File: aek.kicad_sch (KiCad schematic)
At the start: 242 parts, among them J1 Conn_01x04_MountingPin, SW1 SW_Push, U1 ATmega32U4-AU, U2 ATmega32U4-MU, Y1 16MHz

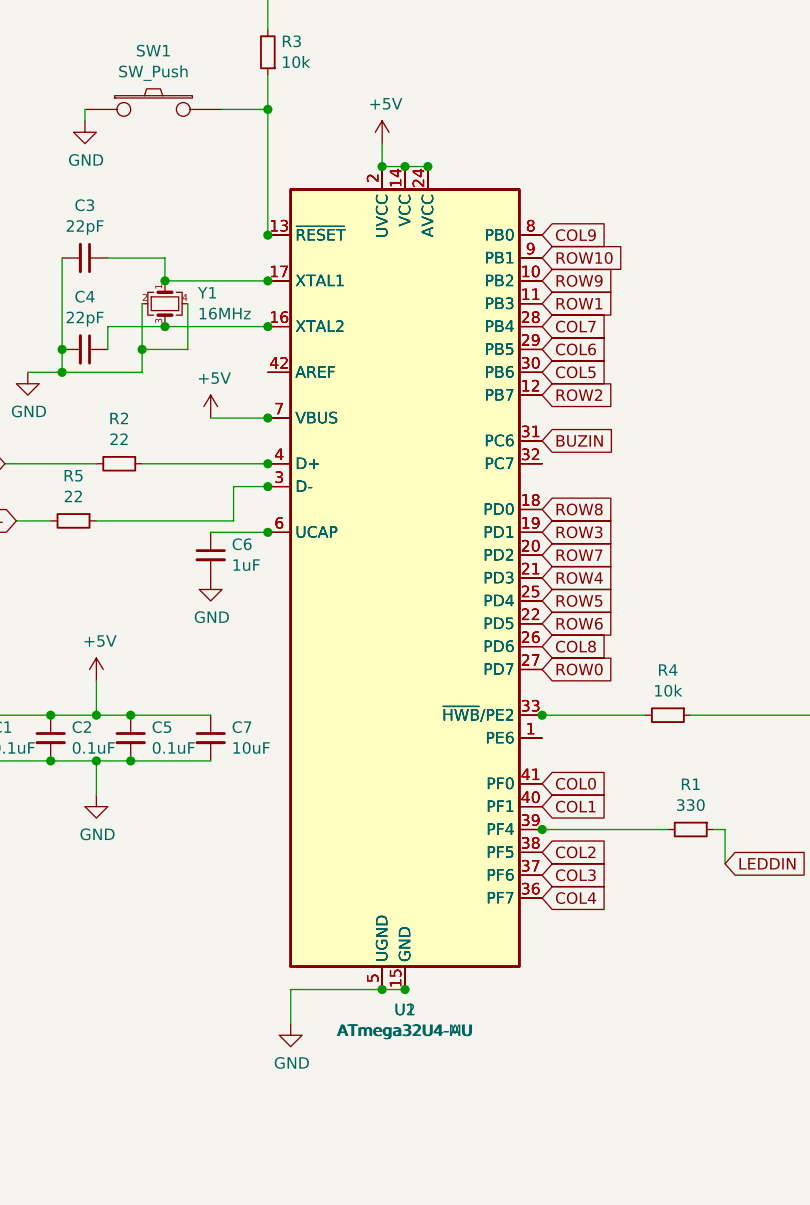
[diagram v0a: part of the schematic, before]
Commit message: cleanup
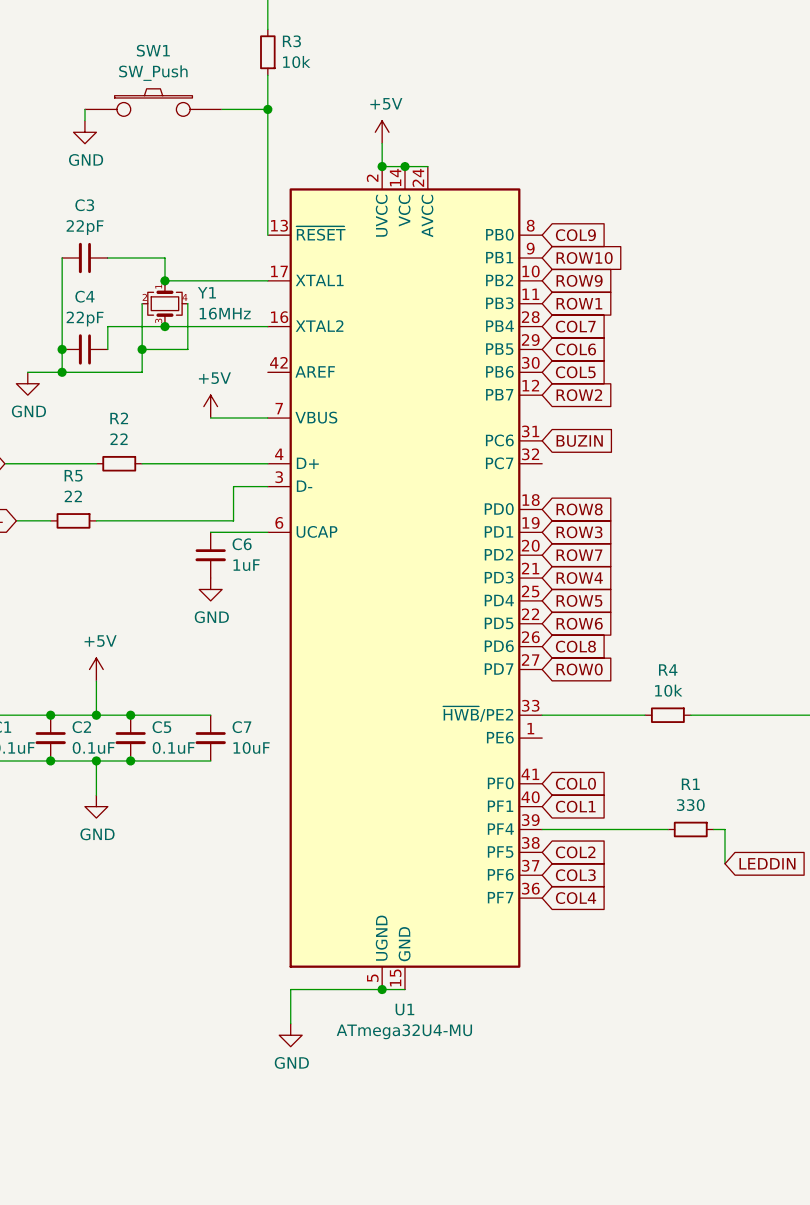
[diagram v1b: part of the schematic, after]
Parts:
- removed U1: ATmega32U4-AU, Package_QFP:TQFP-44_10x10mm_P0.8mm, symbol MCU_Microchip_ATmega:ATmega32U4-AU
- U1: renamed from U2; footprint Package_DFN_QFN:QFN-44-1EP_7x7mm_P0.5mm_EP5.2x5.2mm -> atmega32u4-au-and-mu:atmega32u4-mu-and-au
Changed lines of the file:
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@@
   (junction (at 39.37 59.69) (diameter 1.016) (color 0 0 0 0))
   (junction (at 50.8 35.56) (diameter 1.016) (color 0 0 0 0))
-  (junction (at 50.8 49.53) (diameter 1.016) (color 0 0 0 0))
-  (junction (at 50.8 54.61) (diameter 1.016) (color 0 0 0 0))
-  (junction (at 50.8 59.69) (diameter 1.016) (color 0 0 0 0))
-  (junction (at 50.8 69.85) (diameter 1.016) (color 0 0 0 0))
-  (junction (at 50.8 74.93) (diameter 1.016) (color 0 0 0 0))
-  (junction (at 50.8 77.47) (diameter 1.016) (color 0 0 0 0))
-  (junction (at 50.8 82.55) (diameter 1.016) (color 0 0 0 0))
   (junction (at 63.5 41.91) (diameter 1.016) (color 0 0 0 0))
   (junction (at 63.5 133.35) (diameter 1.016) (color 0 0 0 0))
@@
   (junction (at 64.77 241.3) (diameter 1.016) (color 0 0 0 0))
   (junction (at 66.04 41.91) (diameter 1.016) (color 0 0 0 0))
-  (junction (at 66.04 133.35) (diameter 1.016) (color 0 0 0 0))
-  (junction (at 68.58 41.91) (diameter 1.016) (color 0 0 0 0))
-  (junction (at 81.28 102.87) (diameter 1.016) (color 0 0 0 0))
-  (junction (at 81.28 115.57) (diameter 1.016) (color 0 0 0 0))
   (junction (at 100.33 241.3) (diameter 1.016) (color 0 0 0 0))
   (junction (at 157.48 55.88) (diameter 1.016) (color 0 0 0 0))
@@
     (pin "4")
   )
-  (symbol (lib_id "MCU_Microchip_ATmega:ATmega32U4-AU") (at 66.04 87.63 0) (unit 1)
-    (in_bom yes) (on_board yes)
-    (property "Reference" "U1" (id 0) (at 66.04 135.6106 0))
-    (property "Value" "ATmega32U4-AU" (id 1) (at 66.04 137.922 0))
-    (property "Footprint" "Package_QFP:TQFP-44_10x10mm_P0.8mm" (id 2) (at 66.04 87.63 0)
-      (effects (font (size 1.27 1.27) italic) hide)
-    )
-    (property "Datasheet" "http://ww1.microchip.com/downloads/en/DeviceDoc/Atmel-7766-8-bit-AVR-ATmega16U4-32U4_Datasheet.pdf" (id 3) (at 66.04 87.63 0)
-      (effects (font (size 1.27 1.27)) hide)
-    )
-    (pin "1")
-    (pin "10")
-    (pin "11")
-    (pin "12")
-    (pin "13")
-    (pin "14")
-    (pin "15")
-    (pin "16")
-    (pin "17")
-    (pin "18")
-    (pin "19")
-    (pin "2")
-    (pin "20")
-    (pin "21")
-    (pin "22")
-    (pin "23")
-    (pin "24")
-    (pin "25")
-    (pin "26")
-    (pin "27")
-    (pin "28")
-    (pin "29")
-    (pin "3")
-    (pin "30")
-    (pin "31")
-    (pin "32")
-    (pin "33")
-    (pin "34")
-    (pin "35")
-    (pin "36")
-    (pin "37")
-    (pin "38")
-    (pin "39")
-    (pin "4")
-    (pin "40")
-    (pin "41")
-    (pin "42")
-    (pin "43")
-    (pin "44")
-    (pin "5")
-    (pin "6")
-    (pin "7")
-    (pin "8")
-    (pin "9")
-  )
   (symbol (lib_id "MCU_Microchip_ATmega:ATmega32U4-MU") (at 66.04 87.63 0) (unit 1)
     (in_bom yes) (on_board yes)
-    (property "Reference" "U2" (id 0) (at 66.04 135.6106 0))
+    (property "Reference" "U1" (id 0) (at 66.04 135.6106 0))
     (property "Value" "ATmega32U4-MU" (id 1) (at 66.04 137.922 0))
-    (property "Footprint" "Package_DFN_QFN:QFN-44-1EP_7x7mm_P0.5mm_EP5.2x5.2mm" (id 2) (at 66.04 87.63 0)
+    (property "Footprint" "atmega32u4-au-and-mu:atmega32u4-mu-and-au" (id 2) (at 66.04 87.63 0)
       (effects (font (size 1.27 1.27) italic) hide)
     )
@@
       (reference "SW_Z1") (unit 1) (value "MX-NoLED") (footprint "MX_Alps_Hybrid:MX-1U-NoLED")
     )
-    (path "/00000000-0000-0000-0000-0000611ebb71"
-      (reference "U1") (unit 1) (value "ATmega32U4-AU") (footprint "Package_QFP:TQFP-44_10x10mm_P0.8mm")
-    )
     (path "/2ccdb65d-62ed-42d5-acea-df4cedf22149"
-      (reference "U2") (unit 1) (value "ATmega32U4-MU") (footprint "Package_DFN_QFN:QFN-44-1EP_7x7mm_P0.5mm_EP5.2x5.2mm")
+      (reference "U1") (unit 1) (value "ATmega32U4-MU") (footprint "atmega32u4-au-and-mu:atmega32u4-mu-and-au")
     )
     (path "/00000000-0000-0000-0000-0000612269b2"

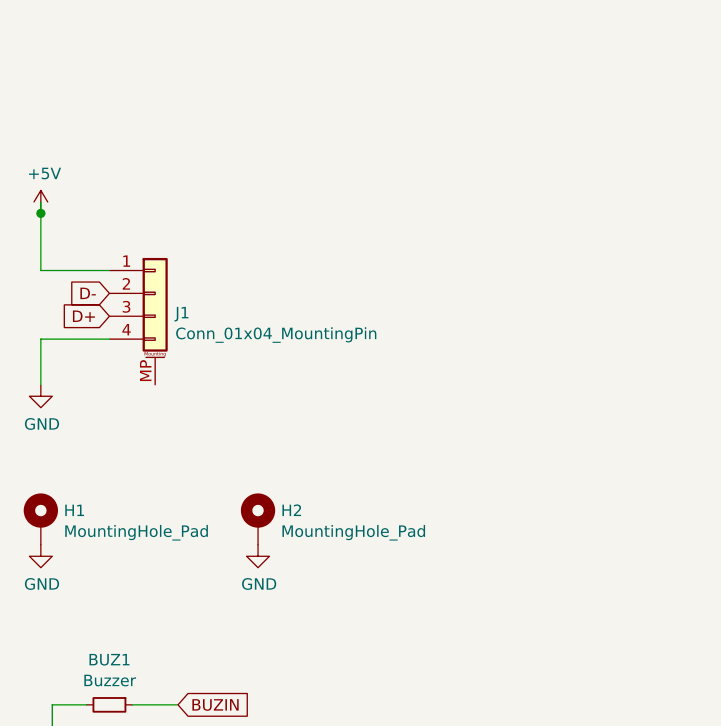
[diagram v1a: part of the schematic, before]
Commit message: bug fixes
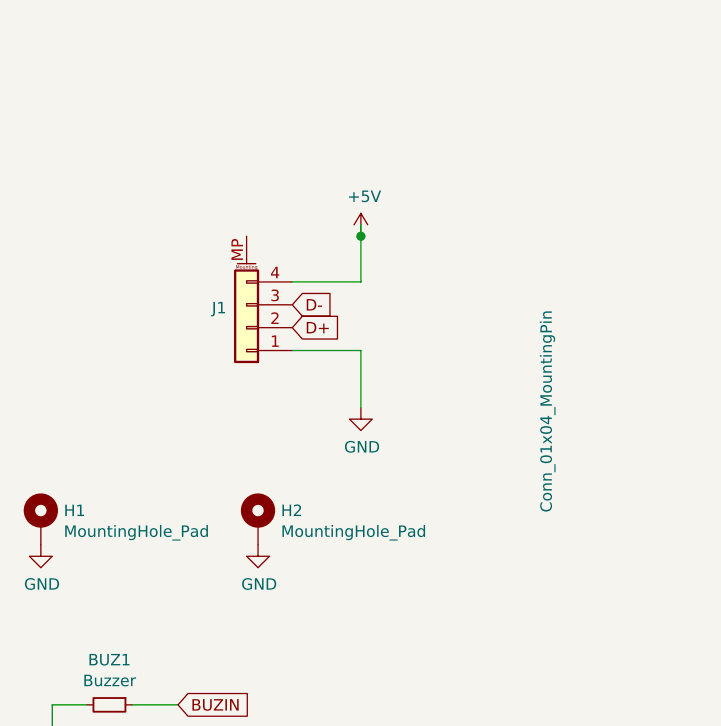
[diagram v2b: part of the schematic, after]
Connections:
- net +5V: now also J1.4 (Pin_4); no longer J1.1 (Pin_1)
- net D+: now also J1.2 (Pin_2); no longer J1.3 (Pin_3)
- net D-: now also J1.3 (Pin_3); no longer J1.2 (Pin_2)
- net GND: now also J1.1 (Pin_1); no longer J1.4 (Pin_4)
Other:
- moved on the sheet: J1
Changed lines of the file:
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@@
 (kicad_sch (version 20210621) (generator eeschema)
   (paper "User" 359.994 359.994)
-  (junction (at 17.78 167.64) (diameter 1.016) (color 0 0 0 0))
   (junction (at 26.67 102.87) (diameter 1.016) (color 0 0 0 0))
   (junction (at 26.67 107.95) (diameter 1.016) (color 0 0 0 0))
@@
   (junction (at 39.37 59.69) (diameter 1.016) (color 0 0 0 0))
   (junction (at 50.8 35.56) (diameter 1.016) (color 0 0 0 0))
+  (junction (at 53.34 170.18) (diameter 1.016) (color 0 0 0 0))
   (junction (at 63.5 41.91) (diameter 1.016) (color 0 0 0 0))
   (junction (at 63.5 133.35) (diameter 1.016) (color 0 0 0 0))
@@
     (stroke (width 0) (type solid) (color 0 0 0 0))
   )
-  (wire (pts (xy 17.78 166.37) (xy 17.78 167.64))
-    (stroke (width 0) (type solid) (color 0 0 0 0))
-  )
-  (wire (pts (xy 17.78 167.64) (xy 17.78 173.99))
-    (stroke (width 0) (type solid) (color 0 0 0 0))
-  )
-  (wire (pts (xy 17.78 181.61) (xy 17.78 186.69))
-    (stroke (width 0) (type solid) (color 0 0 0 0))
-  )
   (wire (pts (xy 19.05 222.25) (xy 19.05 226.06))
     (stroke (width 0) (type solid) (color 0 0 0 0))
@@
     (stroke (width 0) (type solid) (color 0 0 0 0))
   )
-  (wire (pts (xy 25.4 173.99) (xy 17.78 173.99))
-    (stroke (width 0) (type solid) (color 0 0 0 0))
-  )
-  (wire (pts (xy 25.4 181.61) (xy 17.78 181.61))
-    (stroke (width 0) (type solid) (color 0 0 0 0))
-  )
   (wire (pts (xy 26.67 102.87) (xy 31.75 102.87))
     (stroke (width 0) (type solid) (color 0 0 0 0))
@@
     (stroke (width 0) (type solid) (color 0 0 0 0))
   )
+  (wire (pts (xy 45.72 175.26) (xy 53.34 175.26))
+    (stroke (width 0) (type solid) (color 0 0 0 0))
+  )
   (wire (pts (xy 46.99 77.47) (xy 50.8 77.47))
     (stroke (width 0) (type solid) (color 0 0 0 0))
@@
     (stroke (width 0) (type solid) (color 0 0 0 0))
   )
+  (wire (pts (xy 53.34 168.91) (xy 53.34 170.18))
+    (stroke (width 0) (type solid) (color 0 0 0 0))
+  )
+  (wire (pts (xy 53.34 170.18) (xy 53.34 175.26))
+    (stroke (width 0) (type solid) (color 0 0 0 0))
+  )
+  (wire (pts (xy 53.34 182.88) (xy 45.72 182.88))
+    (stroke (width 0) (type solid) (color 0 0 0 0))
+  )
+  (wire (pts (xy 53.34 182.88) (xy 53.34 189.23))
+    (stroke (width 0) (type solid) (color 0 0 0 0))
+  )
   (wire (pts (xy 54.61 259.08) (xy 54.61 254))
     (stroke (width 0) (type solid) (color 0 0 0 0))
@@
     )
   )
-  (global_label "D-" (shape input) (at 25.4 176.53 180) (fields_autoplaced)
-    (effects (font (size 1.27 1.27)) (justify right))
-    (property "Intersheet References" "${INTERSHEET_REFS}" (id 0) (at -12.7 -40.64 0)
-      (effects (font (size 1.27 1.27)) hide)
+  (global_label "BUZIN" (shape input) (at 33.02 222.25 0) (fields_autoplaced)
+    (effects (font (size 1.27 1.27)) (justify left))
+    (property "Intersheet References" "${INTERSHEET_REFS}" (id 0) (at 41.0386 222.1706 0)
+      (effects (font (size 1.27 1.27)) (justify left) hide)
     )
   )
-  (global_label "D+" (shape input) (at 25.4 179.07 180) (fields_autoplaced)
-    (effects (font (size 1.27 1.27)) (justify right))
-    (property "Intersheet References" "${INTERSHEET_REFS}" (id 0) (at -12.7 -40.64 0)
+  (global_label "D-" (shape input) (at 45.72 177.8 0) (fields_autoplaced)
+    (effects (font (size 1.27 1.27)) (justify left))
+    (property "Intersheet References" "${INTERSHEET_REFS}" (id 0) (at 83.82 394.97 0)
       (effects (font (size 1.27 1.27)) hide)
     )
   )
-  (global_label "BUZIN" (shape input) (at 33.02 222.25 0) (fields_autoplaced)
+  (global_label "D+" (shape input) (at 45.72 180.34 0) (fields_autoplaced)
     (effects (font (size 1.27 1.27)) (justify left))
-    (property "Intersheet References" "${INTERSHEET_REFS}" (id 0) (at 41.0386 222.1706 0)
-      (effects (font (size 1.27 1.27)) (justify left) hide)
+    (property "Intersheet References" "${INTERSHEET_REFS}" (id 0) (at 83.82 400.05 0)
+      (effects (font (size 1.27 1.27)) hide)
     )
   )
@@
     )
   )
-  (symbol (lib_id "power:+5V") (at 17.78 167.64 0) (unit 1)
-    (in_bom yes) (on_board yes)
-    (property "Reference" "#PWR0111" (id 0) (at 17.78 171.45 0)
-      (effects (font (size 1.27 1.27)) hide)
-    )
-    (property "Value" "+5V" (id 1) (at 18.161 163.2458 0))
-    (property "Footprint" "" (id 2) (at 17.78 167.64 0)
-      (effects (font (size 1.27 1.27)) hide)
-    )
-    (property "Datasheet" "" (id 3) (at 17.78 167.64 0)
-      (effects (font (size 1.27 1.27)) hide)
-    )
-    (pin "1")
-  )
   (symbol (lib_id "power:+5V") (at 31.75 99.06 0) (unit 1)
     (in_bom yes) (on_board yes)
@@
     (pin "1")
   )
+  (symbol (lib_id "power:+5V") (at 53.34 170.18 0) (unit 1)
+    (in_bom yes) (on_board yes)
+    (property "Reference" "#PWR0111" (id 0) (at 53.34 173.99 0)
+      (effects (font (size 1.27 1.27)) hide)
+    )
+    (property "Value" "+5V" (id 1) (at 53.721 165.7858 0))
+    (property "Footprint" "" (id 2) (at 53.34 170.18 0)
+      (effects (font (size 1.27 1.27)) hide)
+    )
+    (property "Datasheet" "" (id 3) (at 53.34 170.18 0)
+      (effects (font (size 1.27 1.27)) hide)
+    )
+    (pin "1")
+  )
   (symbol (lib_id "power:+5V") (at 63.5 39.37 0) (unit 1)
     (in_bom yes) (on_board yes)
@@
     (pin "1")
   )
-  (symbol (lib_id "power:GND") (at 17.78 186.69 0) (unit 1)
-    (in_bom yes) (on_board yes)
-    (property "Reference" "#PWR0112" (id 0) (at 17.78 193.04 0)
-      (effects (font (size 1.27 1.27)) hide)
-    )
-    (property "Value" "GND" (id 1) (at 17.907 191.0842 0))
-    (property "Footprint" "" (id 2) (at 17.78 186.69 0)
-      (effects (font (size 1.27 1.27)) hide)
-    )
-    (property "Datasheet" "" (id 3) (at 17.78 186.69 0)
-      (effects (font (size 1.27 1.27)) hide)
-    )
-    (pin "1")
-  )
   (symbol (lib_id "power:GND") (at 17.78 204.47 0) (unit 1)
     (in_bom yes) (on_board yes)
@@
     (pin "1")
   )
+  (symbol (lib_id "power:GND") (at 53.34 189.23 0) (unit 1)
+    (in_bom yes) (on_board yes)
+    (property "Reference" "#PWR0112" (id 0) (at 53.34 195.58 0)
+      (effects (font (size 1.27 1.27)) hide)
+    )
+    (property "Value" "GND" (id 1) (at 53.467 193.6242 0))
+    (property "Footprint" "" (id 2) (at 53.34 189.23 0)
+      (effects (font (size 1.27 1.27)) hide)
+    )
+    (property "Datasheet" "" (id 3) (at 53.34 189.23 0)
+      (effects (font (size 1.27 1.27)) hide)
+    )
+    (pin "1")
+  )
   (symbol (lib_id "power:GND") (at 54.61 270.51 0) (unit 1)
     (in_bom yes) (on_board yes)
@@
     (pin "2")
   )
-  (symbol (lib_id "Connector_Generic_MountingPin:Conn_01x04_MountingPin") (at 30.48 176.53 0) (unit 1)
+  (symbol (lib_id "Connector_Generic_MountingPin:Conn_01x04_MountingPin") (at 40.64 180.34 180) (unit 1)
     (in_bom yes) (on_board yes)
-    (property "Reference" "J1" (id 0) (at 32.7152 178.7144 0)
+    (property "Reference" "J1" (id 0) (at 38.4048 178.1556 0)
       (effects (font (size 1.27 1.27)) (justify left))
     )
-    (property "Value" "Conn_01x04_MountingPin" (id 1) (at 32.7152 181.0258 0)
+    (property "Value" "Conn_01x04_MountingPin" (id 1) (at 73.9648 178.3842 90)
       (effects (font (size 1.27 1.27)) (justify left))
     )
-    (property "Footprint" "Connector_JST:JST_SH_SM04B-SRSS-TB_1x04-1MP_P1.00mm_Horizontal" (id 2) (at 30.48 176.53 0)
+    (property "Footprint" "Connector_JST:JST_SH_SM04B-SRSS-TB_1x04-1MP_P1.00mm_Horizontal" (id 2) (at 40.64 180.34 0)
       (effects (font (size 1.27 1.27)) hide)
     )
-    (property "Datasheet" "~" (id 3) (at 30.48 176.53 0)
+    (property "Datasheet" "~" (id 3) (at 40.64 180.34 0)
       (effects (font (size 1.27 1.27)) hide)
     )
